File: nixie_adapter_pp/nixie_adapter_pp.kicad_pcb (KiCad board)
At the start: 2 copper layers, 100 x 38 mm, 6 parts, among them J1 Conn_02x20_Odd_Even, J2 Conn_02x20_Odd_Even

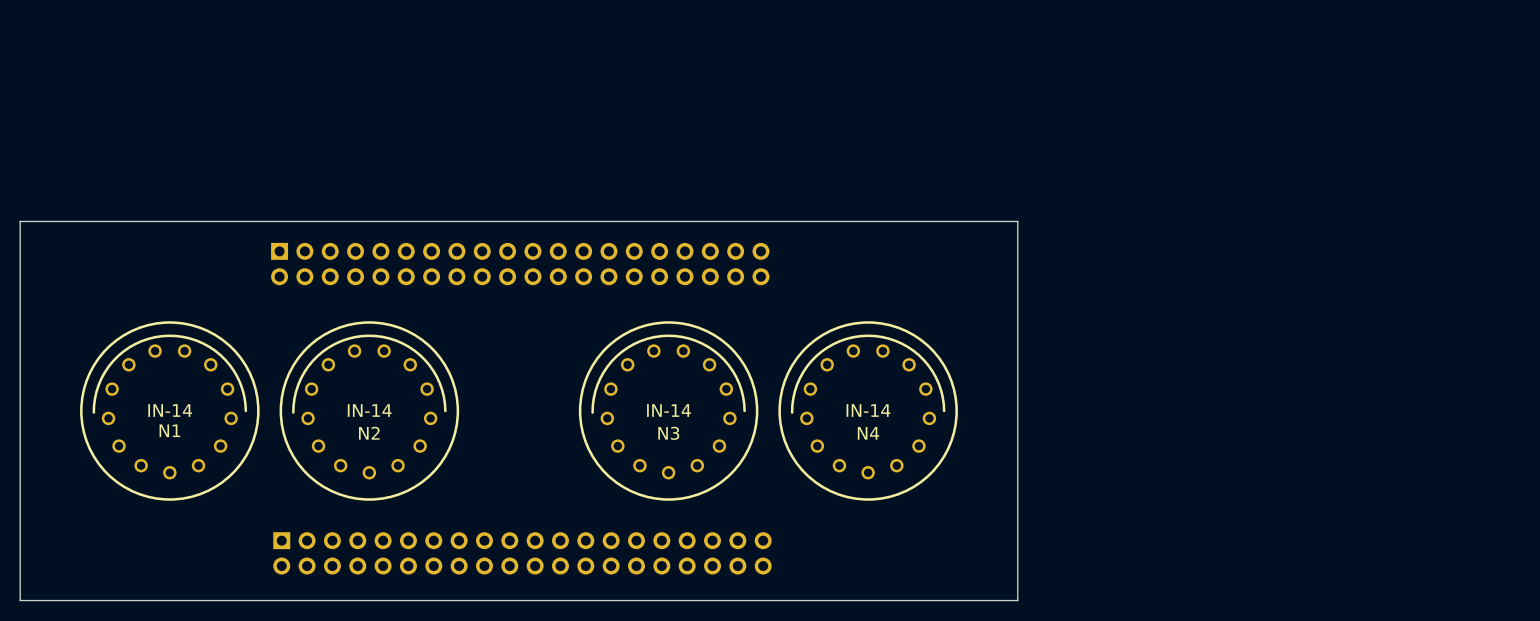
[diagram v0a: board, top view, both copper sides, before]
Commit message: update
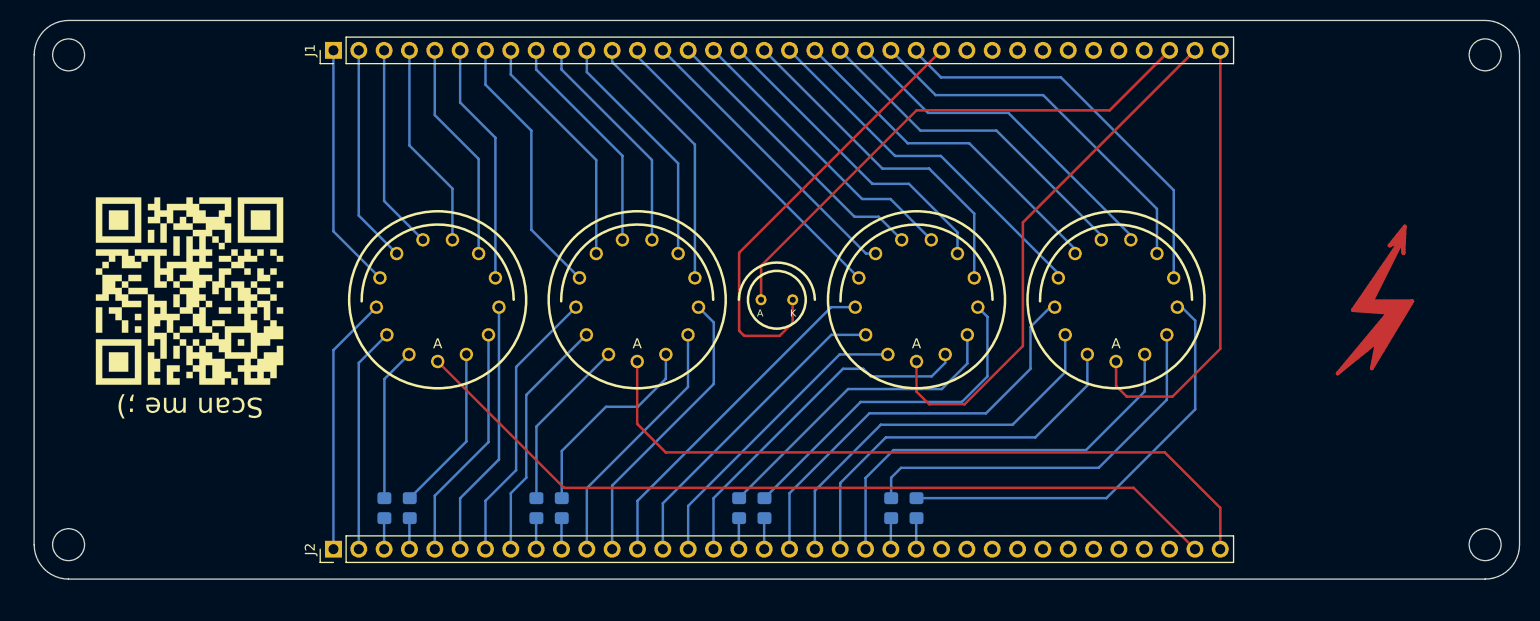
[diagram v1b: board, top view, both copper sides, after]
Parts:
- added G***: LOGO, Espressif:symbol2, F.Cu at (97.0, 82.0)
- added H1: MountingHole, MountingHole:MountingHole_3.2mm_M3, F.Cu at (84.8, 58.3)
- added H2: MountingHole, MountingHole:MountingHole_3.2mm_M3, F.Cu at (226.8, 58.3)
- added H3: MountingHole, MountingHole:MountingHole_3.2mm_M3, F.Cu at (226.8, 107.4)
- added H4: MountingHole, MountingHole:MountingHole_3.2mm_M3, F.Cu at (84.8, 107.4)
- added N5: IN-14, nixies-us:nixies-us-IN-14, F.Cu at (189.8, 82.8)
- added R1: R, Resistor_SMD:R_0805_2012Metric_Pad1.20x1.40mm_HandSolder, B.Cu at (119.0, 103.7)
- added R2: R, Resistor_SMD:R_0805_2012Metric_Pad1.20x1.40mm_HandSolder, B.Cu at (134.3, 103.7)
- added R3: R, Resistor_SMD:R_0805_2012Metric_Pad1.20x1.40mm_HandSolder, B.Cu at (116.5, 103.7)
- added R4: R, Resistor_SMD:R_0805_2012Metric_Pad1.20x1.40mm_HandSolder, B.Cu at (131.7, 103.7)
- added R5: R, Resistor_SMD:R_0805_2012Metric_Pad1.20x1.40mm_HandSolder, B.Cu at (167.3, 103.7)
- added R6: R, Resistor_SMD:R_0805_2012Metric_Pad1.20x1.40mm_HandSolder, B.Cu at (152.1, 103.7)
- added R7: R, Resistor_SMD:R_0805_2012Metric_Pad1.20x1.40mm_HandSolder, B.Cu at (154.6, 103.7)
- added R8: R, Resistor_SMD:R_0805_2012Metric_Pad1.20x1.40mm_HandSolder, B.Cu at (169.8, 103.7)
- added REF**: Symbol_HighVoltage_Type1_CopperTop_Big, Symbol:Symbol_HighVoltage_Type1_CopperTop_Big, F.Cu at (216.4, 83.4)
- J1, J2: value Conn_02x20_Odd_Even -> Conn_01x36; footprint Connector_PinHeader_2.54mm:PinHeader_2x20_P2.54mm_Vertical -> Connector_PinHeader_2.54mm:PinHeader_1x36_P2.54mm_Vertical; moved to F.Cu
- N1: value IN-14 -> IN-3; footprint nixies-us:nixies-us-IN-14 -> nixies-us:nixies-us-IN-3
- moved N1 61.9 mm to (155.8, 82.8)
- moved J1 49.4 mm to (111.4, 57.9), turned to 90 degrees
- moved J2 30.3 mm to (111.4, 107.8), turned to 90 degrees
- moved N2 13.1 mm to (121.8, 82.8)
- moved N4 12.2 mm to (169.8, 82.8)
- moved N3 11.6 mm to (141.8, 82.8)
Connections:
- J1 pad 11: Net-(J1-Pad11) -> Net-(N3-Pad4)
- J1 pad 12: Net-(J1-Pad12) -> Net-(N3-Pad3)
- J1 pad 26: Net-(J1-Pad26) -> unconnected-(J1-Pad26)
- J1 pad 27: Net-(J1-Pad27) -> unconnected-(J1-Pad27)
- J1 pad 28: Net-(J1-Pad28) -> unconnected-(J1-Pad28)
- J1 pad 29: Net-(J1-Pad29) -> unconnected-(J1-Pad29)
- J1 pad 30: Net-(J1-Pad30) -> unconnected-(J1-Pad30)
- J1 pad 31: Net-(J1-Pad31) -> unconnected-(J1-Pad31)
- J1 pad 32: Net-(J1-Pad32) -> unconnected-(J1-Pad32)
- J1 pad 33: Net-(J1-Pad33) -> unconnected-(J1-Pad33)
- J1 pad 35: Net-(J1-Pad35) -> /3_A
- J1 pad 36: Net-(J1-Pad36) -> /4_A
- J2 pad 11: Net-(J2-Pad11) -> Net-(N3-Pad1)
- J2 pad 12: Net-(J2-Pad12) -> Net-(N3-Pad2)
- J2 pad 25: Net-(J2-Pad25) -> unconnected-(J2-Pad25)
- J2 pad 26: Net-(J2-Pad26) -> unconnected-(J2-Pad26)
- J2 pad 27: Net-(J2-Pad27) -> unconnected-(J2-Pad27)
- J2 pad 28: Net-(J2-Pad28) -> unconnected-(J2-Pad28)
- J2 pad 29: Net-(J2-Pad29) -> unconnected-(J2-Pad29)
- J2 pad 30: Net-(J2-Pad30) -> unconnected-(J2-Pad30)
- J2 pad 31: Net-(J2-Pad31) -> unconnected-(J2-Pad31)
- J2 pad 32: Net-(J2-Pad32) -> unconnected-(J2-Pad32)
- J2 pad 33: Net-(J2-Pad33) -> unconnected-(J2-Pad33)
- J2 pad 34: Net-(J2-Pad34) -> unconnected-(J2-Pad34)
- J2 pad 35: Net-(J2-Pad35) -> /1_A
- J2 pad 36: Net-(J2-Pad36) -> /2_A
- J2 pad 8: Net-(J2-Pad8) -> Net-(N3-Pad0)
- N1 pad A: Net-(N1-PadA) -> Net-(J1-Pad34)
- N2 pad 0: Net-(N2-Pad0) -> Net-(J2-Pad2)
- N2 pad 1: Net-(N2-Pad1) -> Net-(J2-Pad5)
- N2 pad 2: Net-(N2-Pad2) -> Net-(J2-Pad6)
- N2 pad 3: Net-(N2-Pad3) -> Net-(J1-Pad6)
- N2 pad 4: Net-(N2-Pad4) -> Net-(J1-Pad5)
- N2 pad 5: Net-(N2-Pad5) -> Net-(J1-Pad4)
- N2 pad 6: Net-(N2-Pad6) -> Net-(J1-Pad3)
- N2 pad 7: Net-(N2-Pad7) -> Net-(J1-Pad2)
- N2 pad 8: Net-(N2-Pad8) -> Net-(J1-Pad1)
- N2 pad 9: Net-(N2-Pad9) -> Net-(J2-Pad1)
- N2 pad A: Net-(N2-PadA) -> /1_A
- N3 pad 5: Net-(N3-Pad5) -> Net-(J1-Pad10)
- N3 pad 6: Net-(N3-Pad6) -> Net-(J1-Pad9)
- N3 pad 7: Net-(N3-Pad7) -> Net-(J1-Pad8)
- N3 pad 8: Net-(N3-Pad8) -> Net-(J1-Pad7)
- N3 pad 9: Net-(N3-Pad9) -> Net-(J2-Pad7)
- N3 pad A: Net-(N3-PadA) -> /2_A
- N4 pad 0: Net-(N4-Pad0) -> Net-(J2-Pad14)
- N4 pad 3: Net-(N4-Pad3) -> Net-(J1-Pad18)
- N4 pad 4: Net-(N4-Pad4) -> Net-(J1-Pad17)
- N4 pad 5: Net-(N4-Pad5) -> Net-(J1-Pad16)
- N4 pad 6: Net-(N4-Pad6) -> Net-(J1-Pad15)
- N4 pad 7: Net-(N4-Pad7) -> Net-(J1-Pad14)
- N4 pad 8: Net-(N4-Pad8) -> Net-(J1-Pad13)
- N4 pad 9: Net-(N4-Pad9) -> Net-(J2-Pad13)
- N4 pad A: Net-(N4-PadA) -> /3_A
- N4 pad LHDP: Net-(N4-PadLHDP) -> Net-(J2-Pad16)
- N4 pad RHDP: Net-(N4-PadRHDP) -> Net-(J2-Pad15)
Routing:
- net /1_A: track 0.00 -> 83.7 mm
- net /2_A: track 0.00 -> 72.3 mm
- net /3_A: track 0.00 -> 53.4 mm
- net Net-(J1-Pad34): track 0.00 -> 53.3 mm
- net /4_A: track 0.00 -> 45.7 mm
- net Net-(J1-Pad25): track 0.00 -> 44.9 mm
- net Net-(N5-Pad2): track 0.00 -> 43.1 mm
- net Net-(N5-PadLHDP): track 0.00 -> 42.9 mm
- net Net-(J2-Pad19): track 0.00 -> 42.6 mm
- net Net-(J1-Pad24): track 0.00 -> 40.1 mm
- net Net-(J2-Pad20): track 0.00 -> 40.1 mm
- net Net-(R5-Pad1): track 0.00 -> 39.9 mm
- net Net-(J2-Pad21): track 0.00 -> 39.0 mm
- net Net-(J1-Pad23): track 0.00 -> 37.3 mm
- net Net-(J1-Pad19): track 0.00 -> 36.2 mm
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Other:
- board size 100 x 38 mm -> 148.9 x 56 mm
- net class Default removed
- board text added: "A"
- board text added: "K"
- board text added: "Scan me ;)"
